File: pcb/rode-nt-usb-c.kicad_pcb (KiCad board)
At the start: 2 copper layers, 36 x 15 mm, 6 parts, among them J1 USB_C_Receptacle_USB2.0_16P, J2 Conn_01x05_Pin

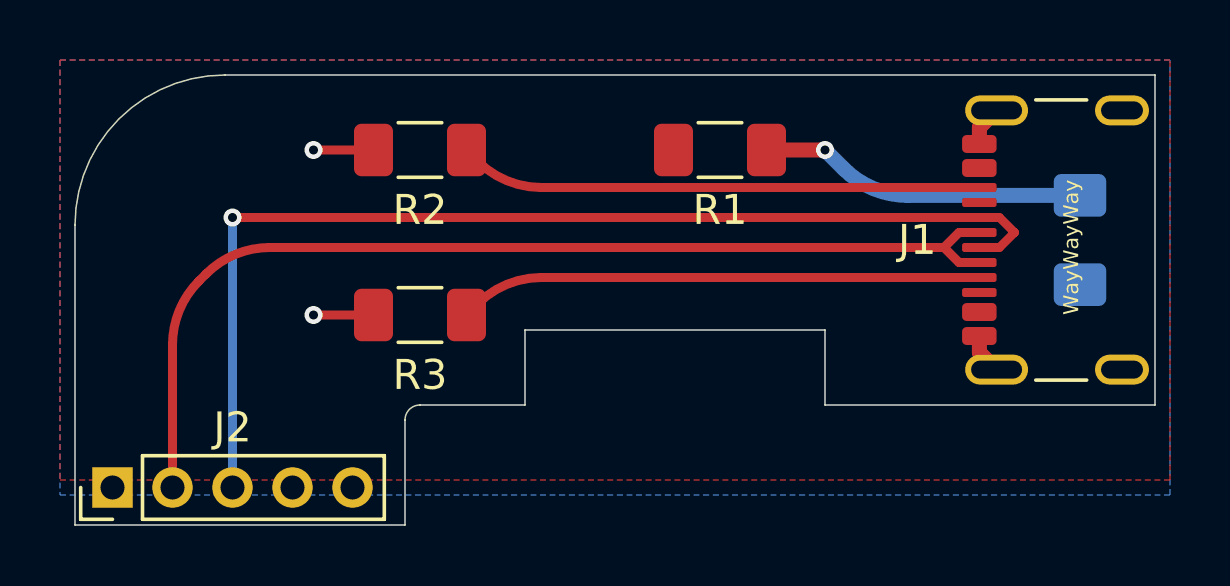
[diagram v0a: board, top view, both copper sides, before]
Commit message: Update design
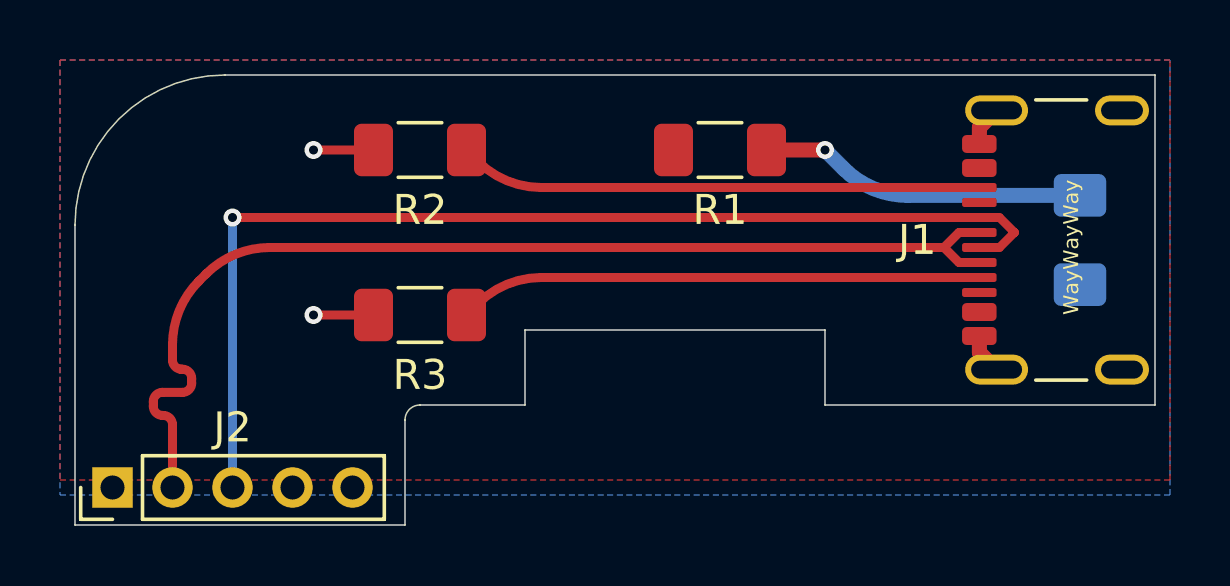
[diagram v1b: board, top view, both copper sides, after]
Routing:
- net D-: track 35.0 -> 36.7 mm
- net Net-(J1-CC2): track 17.5 -> 16.9 mm
- net Net-(J1-CC1): track 17.5 -> 16.9 mm
